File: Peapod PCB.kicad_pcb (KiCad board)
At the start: 2 copper layers, 16 parts, among them J1 CONN_01X01, J2 CONN_01X02, J3 CONN_01X06, J5 CONN_01X01, J6 CONN_01X01, J7 CONN_01X02, U1 ESP8266

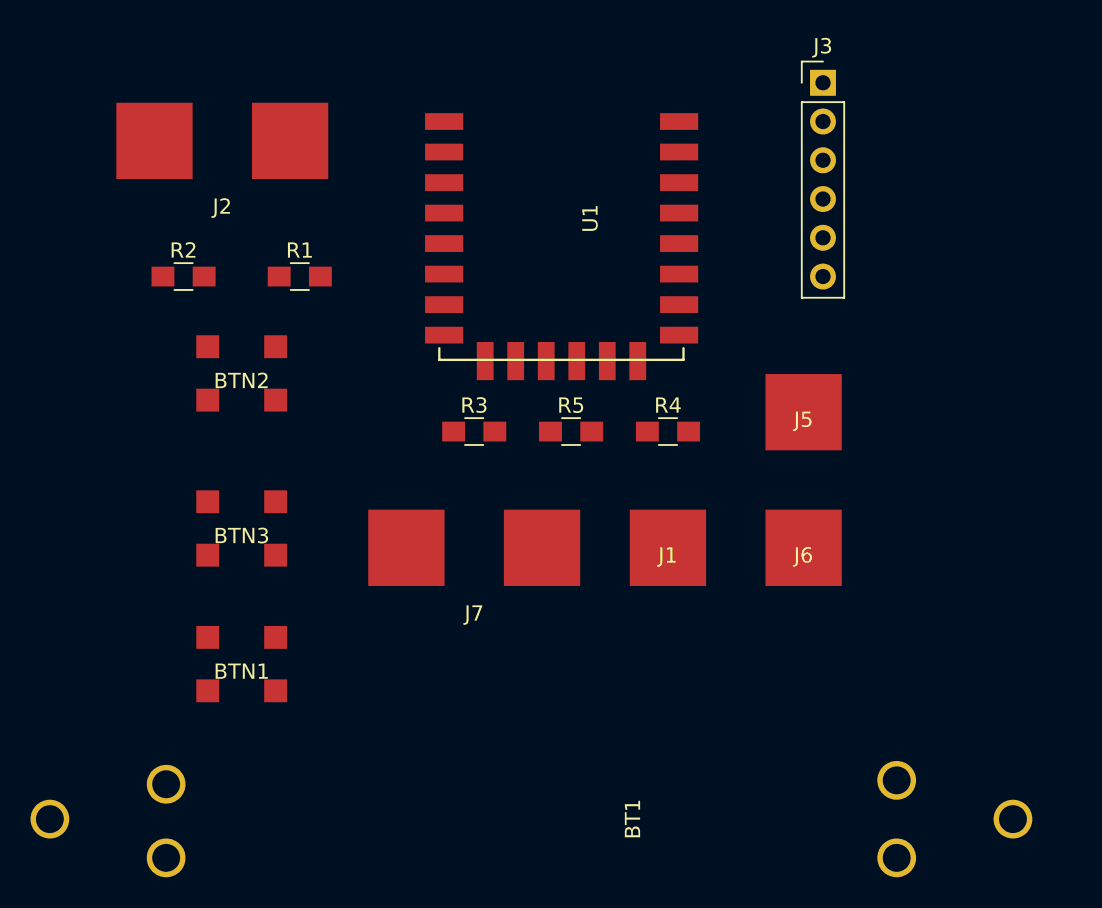
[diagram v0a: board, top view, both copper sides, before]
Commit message: Changed main file for layout
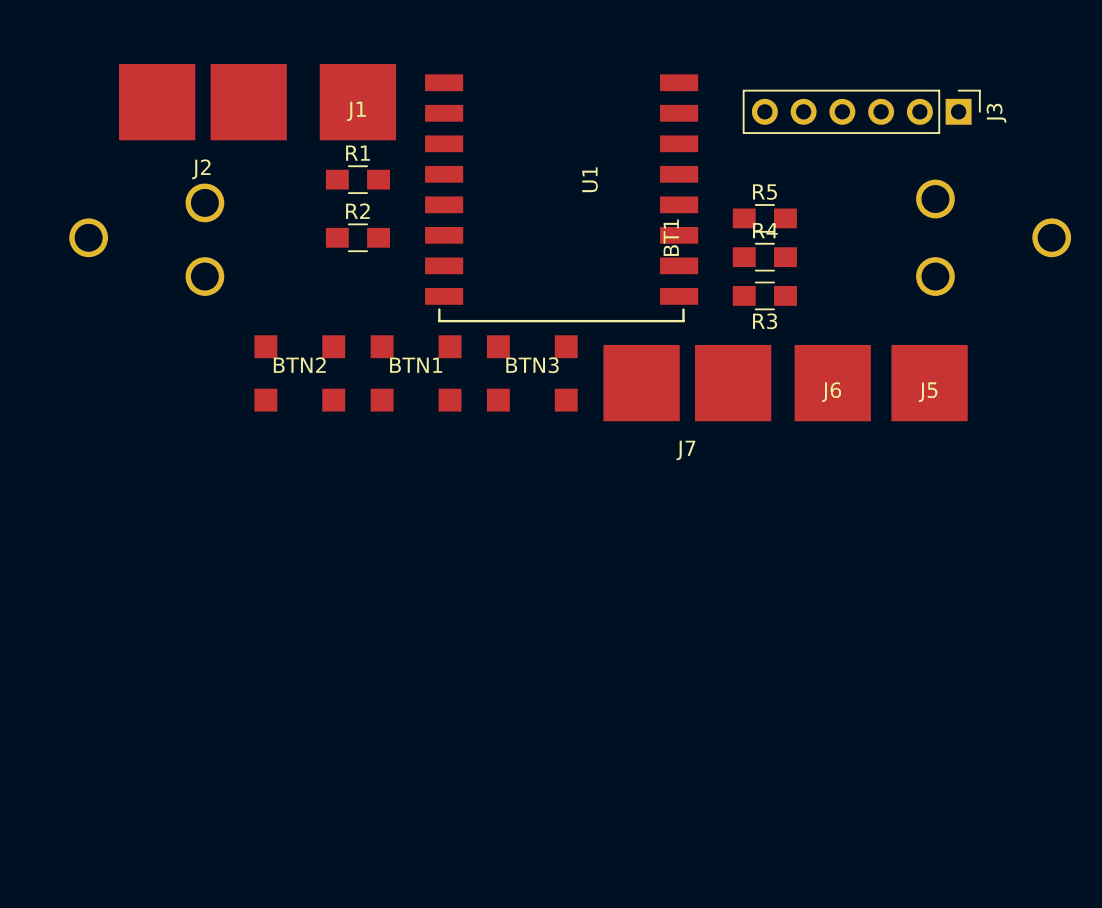
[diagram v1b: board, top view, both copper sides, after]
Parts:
- moved BT1 38.2 mm to (193.0, 39.4)
- moved J1 35.6 mm to (179.1, 30.5)
- moved BTN1 22.2 mm to (182.9, 48.3), turned to 180 degrees
- moved BTN3 21.6 mm to (190.5, 48.3), turned to 180 degrees
- moved R3 21.0 mm to (205.7, 43.2), turned to 180 degrees
- moved R5 18.9 mm to (205.7, 38.1)
- moved J7 17.7 mm to (200.7, 48.9)
- moved R4 13.1 mm to (205.7, 40.6)
- moved R2 11.7 mm to (179.1, 39.4)
- moved J6 11.0 mm to (210.2, 48.9)
- moved J3 9.09 mm to (218.4, 31.1), turned to 270 degrees
- moved J5 8.47 mm to (216.5, 48.9)
- moved R1 7.41 mm to (179.1, 35.6)
- moved BTN2 3.81 mm to (175.3, 48.3), turned to 180 degrees
- moved J2 2.84 mm to (168.9, 30.5)
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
